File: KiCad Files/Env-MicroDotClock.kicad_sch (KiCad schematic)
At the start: 48 parts, among them IC1 IS31FL3730-QFLS2-TR, IC2 IS31FL3730-QFLS2-TR, IC3 IS31FL3730-QFLS2-TR, IC4 IS31FL3730-QFLS2-TR, J1 Conn_01x06_Pin, M1 Dip-14 Socket, M2 Dip-14 Socket, M3 Dip-14 Socket, M4 Dip-14 Socket, M5 Dip-14 Socket, M6 Dip-14 Socket, M7 Dip-14 Socket, M8 Dip-14 Socket, Q1 2SC1815, SW1 SKRK, SW2 SKRK, SW3 SKRK, SW4 SKRK, U1 Raspberry Pi Pico, U3 DS3231M

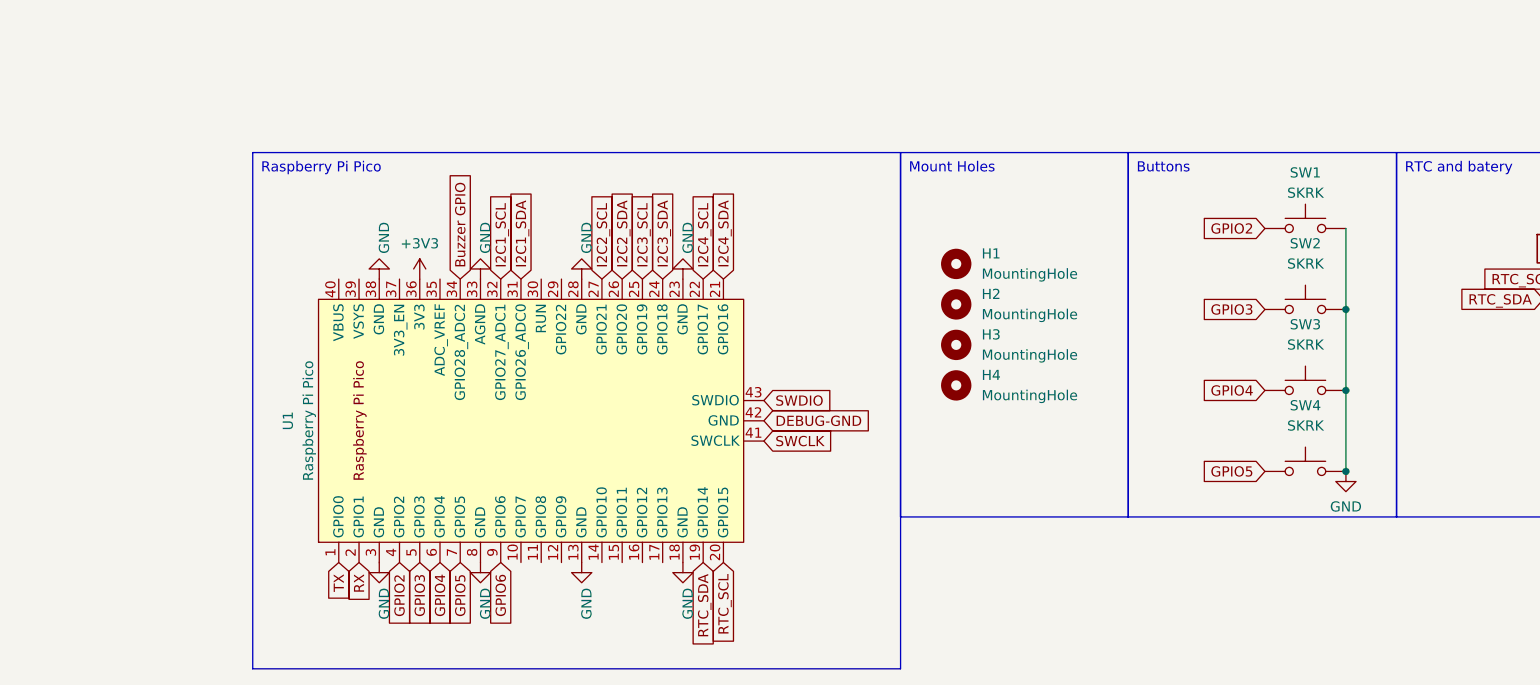
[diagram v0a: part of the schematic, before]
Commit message: added more buttons, re-worked some bits and pieces here and there.
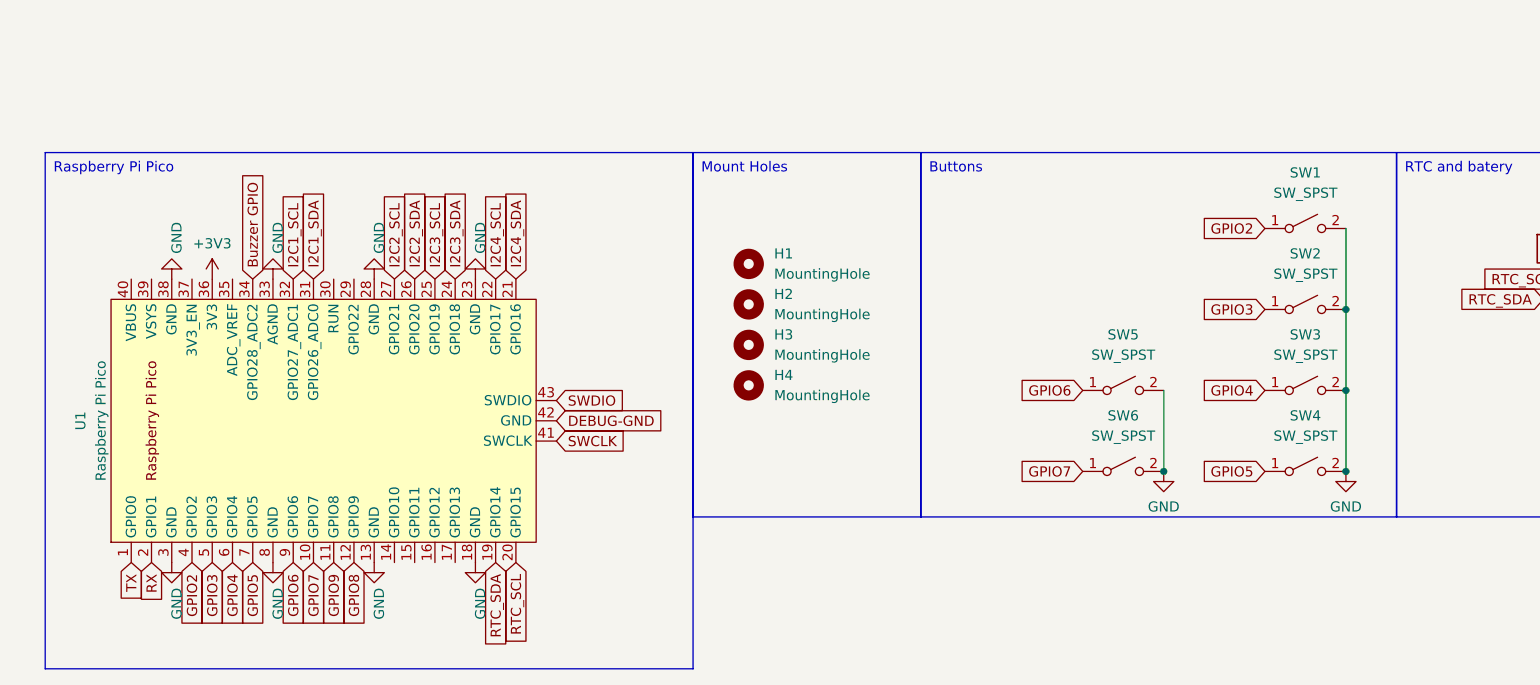
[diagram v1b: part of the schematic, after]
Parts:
- removed SW1, SW2, SW3, SW4: SKRK, Button_Switch_SMD:SW_Push_SPST_NO_Alps_SKRK, symbol Switch:SW_Push
- added SW1, SW2, SW3, SW4, SW5, SW6: SW_SPST, Button_Switch_SMD:SW_Push_SPST_NO_Alps_SKRK, symbol Switch:SW_SPST
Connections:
- net GND: now also SW1.2 (B), SW2.2 (B), SW3.2 (B), SW4.2 (B), SW5.2 (B), SW6.2 (B)
- net GPIO2: now also SW1.1 (A)
- net GPIO3: now also SW2.1 (A)
- net GPIO4: now also SW3.1 (A)
- net GPIO5: now also SW4.1 (A)
- net GPIO6: now also SW5.1 (A)
- net GPIO7: now reaches U1.10 (GPIO7)
- net GPIO7: now also SW6.1 (A)
- net GPIO9: now reaches U1.11 (GPIO8)
- net GPIO8: now reaches U1.12 (GPIO9)
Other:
- moved on the sheet: H1, H2, H3, H4, U1
